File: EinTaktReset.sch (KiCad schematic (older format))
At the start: 36 parts

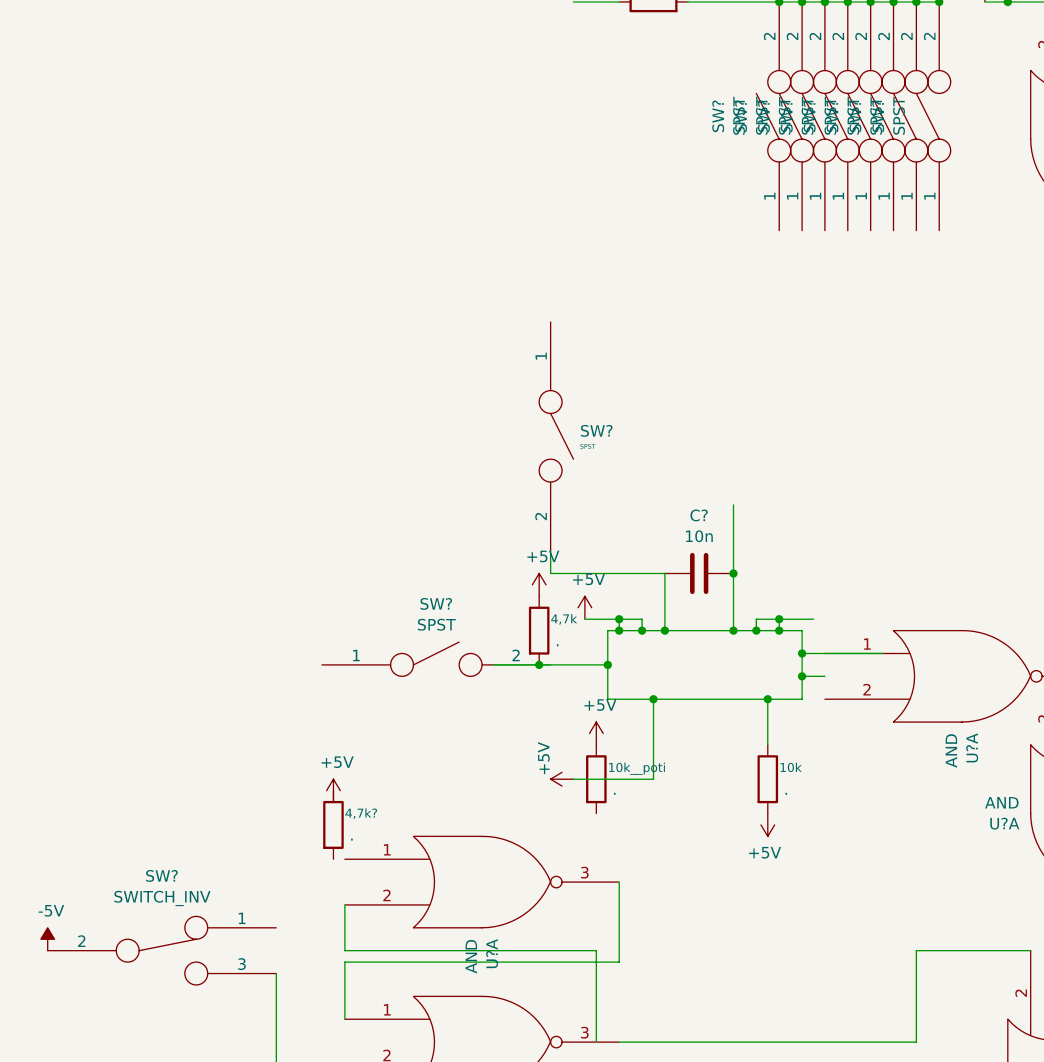
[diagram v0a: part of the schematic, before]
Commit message: added lib
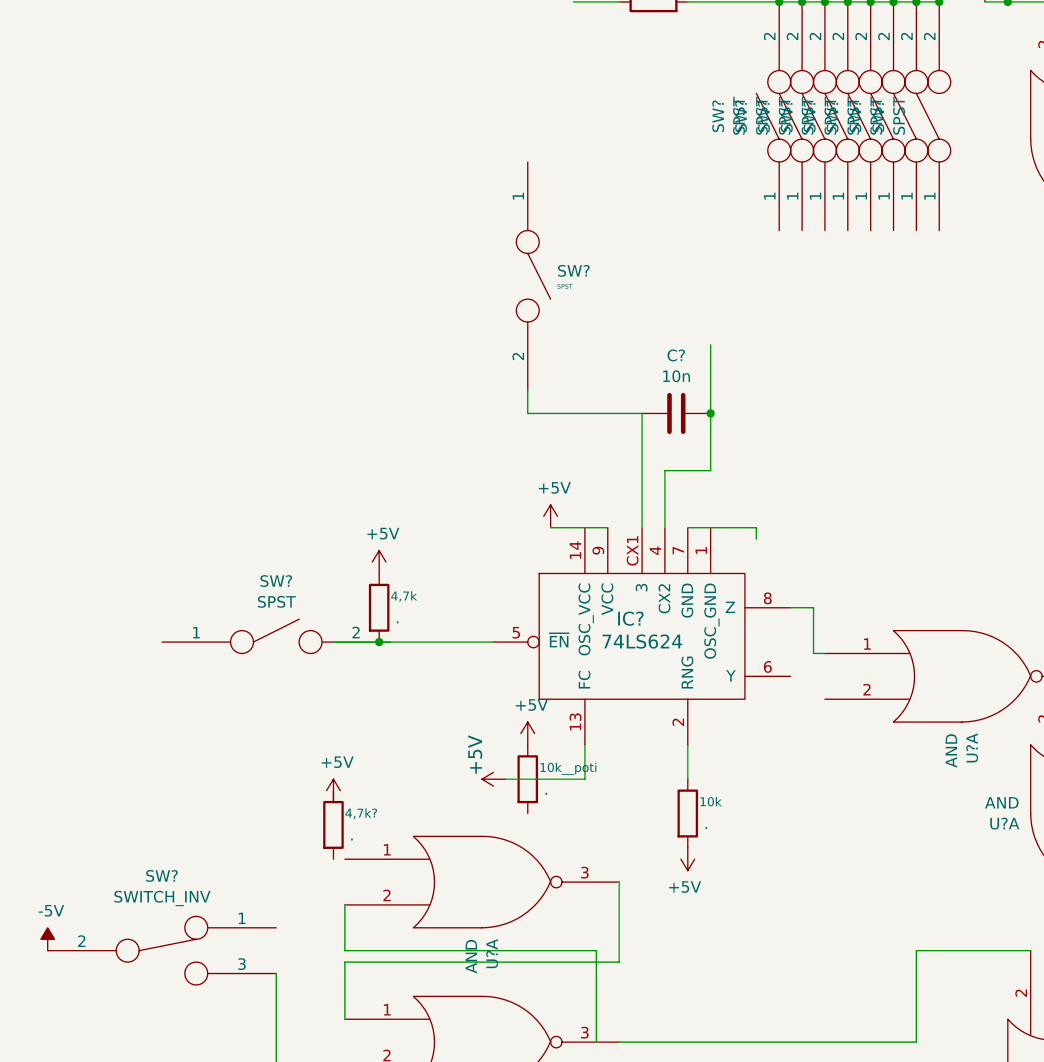
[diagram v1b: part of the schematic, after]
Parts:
- added IC?: 74LS624, symbol 74LS624
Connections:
- wire segments 41 -> 37
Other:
- moved on the sheet: 10k, 10k__poti, 4,7k, C?, SW?
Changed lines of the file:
@@
 LIBS:contrib
 LIBS:valves
+LIBS:vco
 LIBS:EinTaktReset-cache
 EELAYER 25 0
@@
 	0    1    1    0
 $EndComp
-Wire Wire Line
-	3100 5050 3100 4500
 $Comp
 L C C?
 U 1 1 57E97853
-P 2950 4800
-F 0 "C?" V 2698 4800 50  0000 C CNN
-F 1 "10n" V 2789 4800 50  0000 C CNN
-F 2 "" H 2988 4650 50  0000 C CNN
-F 3 "" H 2950 4800 50  0000 C CNN
-	1    2950 4800
-	0    1    1    0
-$EndComp
-Wire Wire Line
-	2800 4800 2300 4800
-Wire Wire Line
-	2300 4800 2300 4700
-Connection ~ 3100 4800
-Wire Wire Line
-	2800 5050 2800 4800
+P 2850 4100
+F 0 "C?" V 2598 4100 50  0000 C CNN
+F 1 "10n" V 2689 4100 50  0000 C CNN
+F 2 "" H 2888 3950 50  0000 C CNN
+F 3 "" H 2850 4100 50  0000 C CNN
+	1    2850 4100
+	0    1    1    0
+$EndComp
+Wire Wire Line
+	2200 4100 2200 4000
 $Comp
 L SPST SW?
 U 1 1 57E97A95
-P 2300 4200
-F 0 "SW?" V 2278 4328 50  0000 L CNN
-F 1 "SPST" V 2345 4328 20  0000 L CNN
-F 2 "" H 2300 4200 50  0000 C CNN
-F 3 "" H 2300 4200 50  0000 C CNN
-	1    2300 4200
+P 2200 3500
+F 0 "SW?" V 2178 3628 50  0000 L CNN
+F 1 "SPST" V 2245 3628 20  0000 L CNN
+F 2 "" H 2200 3500 50  0000 C CNN
+F 3 "" H 2200 3500 50  0000 C CNN
+	1    2200 3500
 	0    1    1    0
 $EndComp
@@
 	5850 4350 5850 5150
 Wire Wire Line
-	2550 5050 3400 5050
-Wire Wire Line
-	3400 5050 3400 5350
-Connection ~ 3100 5050
-Wire Wire Line
-	3400 5350 2550 5350
-Wire Wire Line
-	2550 5350 2550 5050
-Connection ~ 2800 5050
-Wire Wire Line
-	2700 5000 2700 5050
-Wire Wire Line
-	2450 5000 2700 5000
-Connection ~ 2700 5050
-Wire Wire Line
-	2600 5050 2600 5000
-Connection ~ 2600 5000
-Connection ~ 2600 5050
-Wire Wire Line
-	3200 5050 3200 5000
-Wire Wire Line
-	3200 5000 3450 5000
-Connection ~ 3200 5050
-Wire Wire Line
-	3300 5000 3300 5050
-Connection ~ 3300 5050
-Connection ~ 3300 5000
-Wire Wire Line
-	3400 5150 3750 5150
-Connection ~ 3400 5150
-Wire Wire Line
-	3400 5250 3500 5250
-Connection ~ 3400 5250
-Wire Wire Line
-	3250 5350 3250 5550
-Connection ~ 3250 5350
-Wire Wire Line
-	2750 5350 2750 5700
-Connection ~ 2750 5350
-Wire Wire Line
-	2050 5200 2550 5200
-Connection ~ 2550 5200
+	2300 4600 2550 4600
+Wire Wire Line
+	1350 5100 2050 5100
 $Comp
 L R 4,7k
 U 1 1 5845B97A
-P 2250 5050
-F 0 "4,7k" H 2300 5100 39  0000 L CNN
-F 1 "." H 2320 5005 50  0000 L CNN
-F 2 "" V 2180 5050 50  0000 C CNN
-F 3 "" H 2250 5050 50  0000 C CNN
-	1    2250 5050
-	1    0    0    -1
-$EndComp
-Connection ~ 2250 5200
+P 1550 4950
+F 0 "4,7k" H 1600 5000 39  0000 L CNN
+F 1 "." H 1620 4905 50  0000 L CNN
+F 2 "" V 1480 4950 50  0000 C CNN
+F 3 "" H 1550 4950 50  0000 C CNN
+	1    1550 4950
+	1    0    0    -1
+$EndComp
+Connection ~ 1550 5100
 $Comp
 L SPST SW?
 U 1 1 5845BEEF
-P 1800 5200
-F 0 "SW?" H 1800 5465 50  0000 C CNN
-F 1 "SPST" H 1800 5374 50  0000 C CNN
-F 2 "" H 1800 5200 50  0000 C CNN
-F 3 "" H 1800 5200 50  0000 C CNN
-	1    1800 5200
+P 1100 5100
+F 0 "SW?" H 1100 5365 50  0000 C CNN
+F 1 "SPST" H 1100 5274 50  0000 C CNN
+F 2 "" H 1100 5100 50  0000 C CNN
+F 3 "" H 1100 5100 50  0000 C CNN
+	1    1100 5100
 	1    0    0    -1
 $EndComp
@@
 L R 10k
 U 1 1 5845CFFB
-P 3250 5700
-F 0 "10k" H 3300 5750 39  0000 L CNN
-F 1 "." H 3320 5655 50  0000 L CNN
-F 2 "" V 3180 5700 50  0000 C CNN
-F 3 "" H 3250 5700 50  0000 C CNN
-	1    3250 5700
+P 2900 5850
+F 0 "10k" H 2950 5900 39  0000 L CNN
+F 1 "." H 2970 5805 50  0000 L CNN
+F 2 "" V 2830 5850 50  0000 C CNN
+F 3 "" H 2900 5850 50  0000 C CNN
+	1    2900 5850
 	1    0    0    -1
 $EndComp
@@
 L R 10k__poti
 U 1 1 5845D124
-P 2500 5700
-F 0 "10k__poti" H 2550 5750 39  0000 L CNN
-F 1 "." H 2570 5655 50  0000 L CNN
-F 2 "" V 2430 5700 50  0000 C CNN
-F 3 "" H 2500 5700 50  0000 C CNN
-	1    2500 5700
-	1    0    0    -1
-$EndComp
-Wire Wire Line
-	2750 5700 2400 5700
+P 2200 5700
+F 0 "10k__poti" H 2250 5750 39  0000 L CNN
+F 1 "." H 2270 5655 50  0000 L CNN
+F 2 "" V 2130 5700 50  0000 C CNN
+F 3 "" H 2200 5700 50  0000 C CNN
+	1    2200 5700
+	1    0    0    -1
+$EndComp
+Wire Wire Line
+	2450 5700 2100 5700
 $Comp
 L +5V #PWR?
 U 1 1 5845D52B
-P 2400 5700
-F 0 "#PWR?" H 2400 5550 50  0001 C CNN
-F 1 "+5V" H 2415 5828 0   0000 L CNN
-F 2 "" H 2400 5700 50  0000 C CNN
-F 3 "" H 2400 5700 50  0000 C CNN
-	1    2400 5700
+P 2100 5700
+F 0 "#PWR?" H 2100 5550 50  0001 C CNN
+F 1 "+5V" H 2115 5828 60  0000 L CNN
+F 2 "" H 2100 5700 50  0000 C CNN
+F 3 "" H 2100 5700 50  0000 C CNN
+	1    2100 5700
 	0    -1   -1   0
 $EndComp
@@
 L +5V #PWR?
 U 1 1 5845DB56
-P 2500 5550
-F 0 "#PWR?" H 2500 5400 50  0001 C CNN
-F 1 "+5V" H 2515 5723 50  0000 C CNN
-F 2 "" H 2500 5550 50  0000 C CNN
-F 3 "" H 2500 5550 50  0000 C CNN
-	1    2500 5550
+P 2200 5550
+F 0 "#PWR?" H 2200 5400 50  0001 C CNN
+F 1 "+5V" H 2215 5723 50  0000 C CNN
+F 2 "" H 2200 5550 50  0000 C CNN
+F 3 "" H 2200 5550 50  0000 C CNN
+	1    2200 5550
 	1    0    0    -1
 $EndComp
@@
 L +5V #PWR?
 U 1 1 5845DBA0
-P 2250 4900
-F 0 "#PWR?" H 2250 4750 50  0001 C CNN
-F 1 "+5V" H 2265 5073 50  0000 C CNN
-F 2 "" H 2250 4900 50  0000 C CNN
-F 3 "" H 2250 4900 50  0000 C CNN
-	1    2250 4900
+P 1550 4800
+F 0 "#PWR?" H 1550 4650 50  0001 C CNN
+F 1 "+5V" H 1565 4973 50  0000 C CNN
+F 2 "" H 1550 4800 50  0000 C CNN
+F 3 "" H 1550 4800 50  0000 C CNN
+	1    1550 4800
 	1    0    0    -1
 $EndComp
@@
 L +5V #PWR?
 U 1 1 5845DBEA
-P 2450 5000
-F 0 "#PWR?" H 2450 4850 50  0001 C CNN
-F 1 "+5V" H 2465 5173 50  0000 C CNN
-F 2 "" H 2450 5000 50  0000 C CNN
-F 3 "" H 2450 5000 50  0000 C CNN
-	1    2450 5000
+P 2300 4600
+F 0 "#PWR?" H 2300 4450 50  0001 C CNN
+F 1 "+5V" H 2315 4773 50  0000 C CNN
+F 2 "" H 2300 4600 50  0000 C CNN
+F 3 "" H 2300 4600 50  0000 C CNN
+	1    2300 4600
 	1    0    0    -1
 $EndComp
@@
 L +5V #PWR?
 U 1 1 5845DC34
-P 3250 5850
-F 0 "#PWR?" H 3250 5700 50  0001 C CNN
-F 1 "+5V" H 3265 6023 50  0000 C CNN
-F 2 "" H 3250 5850 50  0000 C CNN
-F 3 "" H 3250 5850 50  0000 C CNN
-	1    3250 5850
+P 2900 6000
+F 0 "#PWR?" H 2900 5850 50  0001 C CNN
+F 1 "+5V" H 2915 6173 50  0000 C CNN
+F 2 "" H 2900 6000 50  0000 C CNN
+F 3 "" H 2900 6000 50  0000 C CNN
+	1    2900 6000
 	-1   0    0    1
 $EndComp
@@
 Text GLabel 7600 1800 0    60   Input ~ 0
 en-ln1
+$Comp
+L 74LS624 IC?
+U 1 1 5A158E16
+P 2700 5100
+F 0 "IC?" H 2650 5200 60  0000 C CNN
+F 1 "74LS624" H 2700 5100 60  0000 C CNN
+F 2 "" H 2700 5100 60  0001 C CNN
+F 3 "" H 2700 5100 60  0001 C CNN
+	1    2700 5100
+	1    0    0    -1
+$EndComp
+Wire Wire Line
+	2700 4100 2700 4600
+Connection ~ 3000 4100
+Wire Wire Line
+	2700 4100 2200 4100
+Wire Wire Line
+	3000 4350 3000 3800
+Wire Wire Line
+	3000 4350 2800 4350
+Wire Wire Line
+	2800 4350 2800 4600
+Wire Wire Line
+	3350 4950 3450 4950
+Wire Wire Line
+	3450 4950 3450 5150
+Wire Wire Line
+	3450 5150 3500 5150
+Wire Wire Line
+	2900 4600 3200 4600
+Wire Wire Line
+	3200 4600 3200 4650
+Wire Wire Line
+	2450 5700 2450 5550
+Wire Wire Line
+	2900 5550 2900 5700
 $EndSCHEMATC
